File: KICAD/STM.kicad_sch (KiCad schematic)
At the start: 1 part, among them IC5 STM32F746BGT6

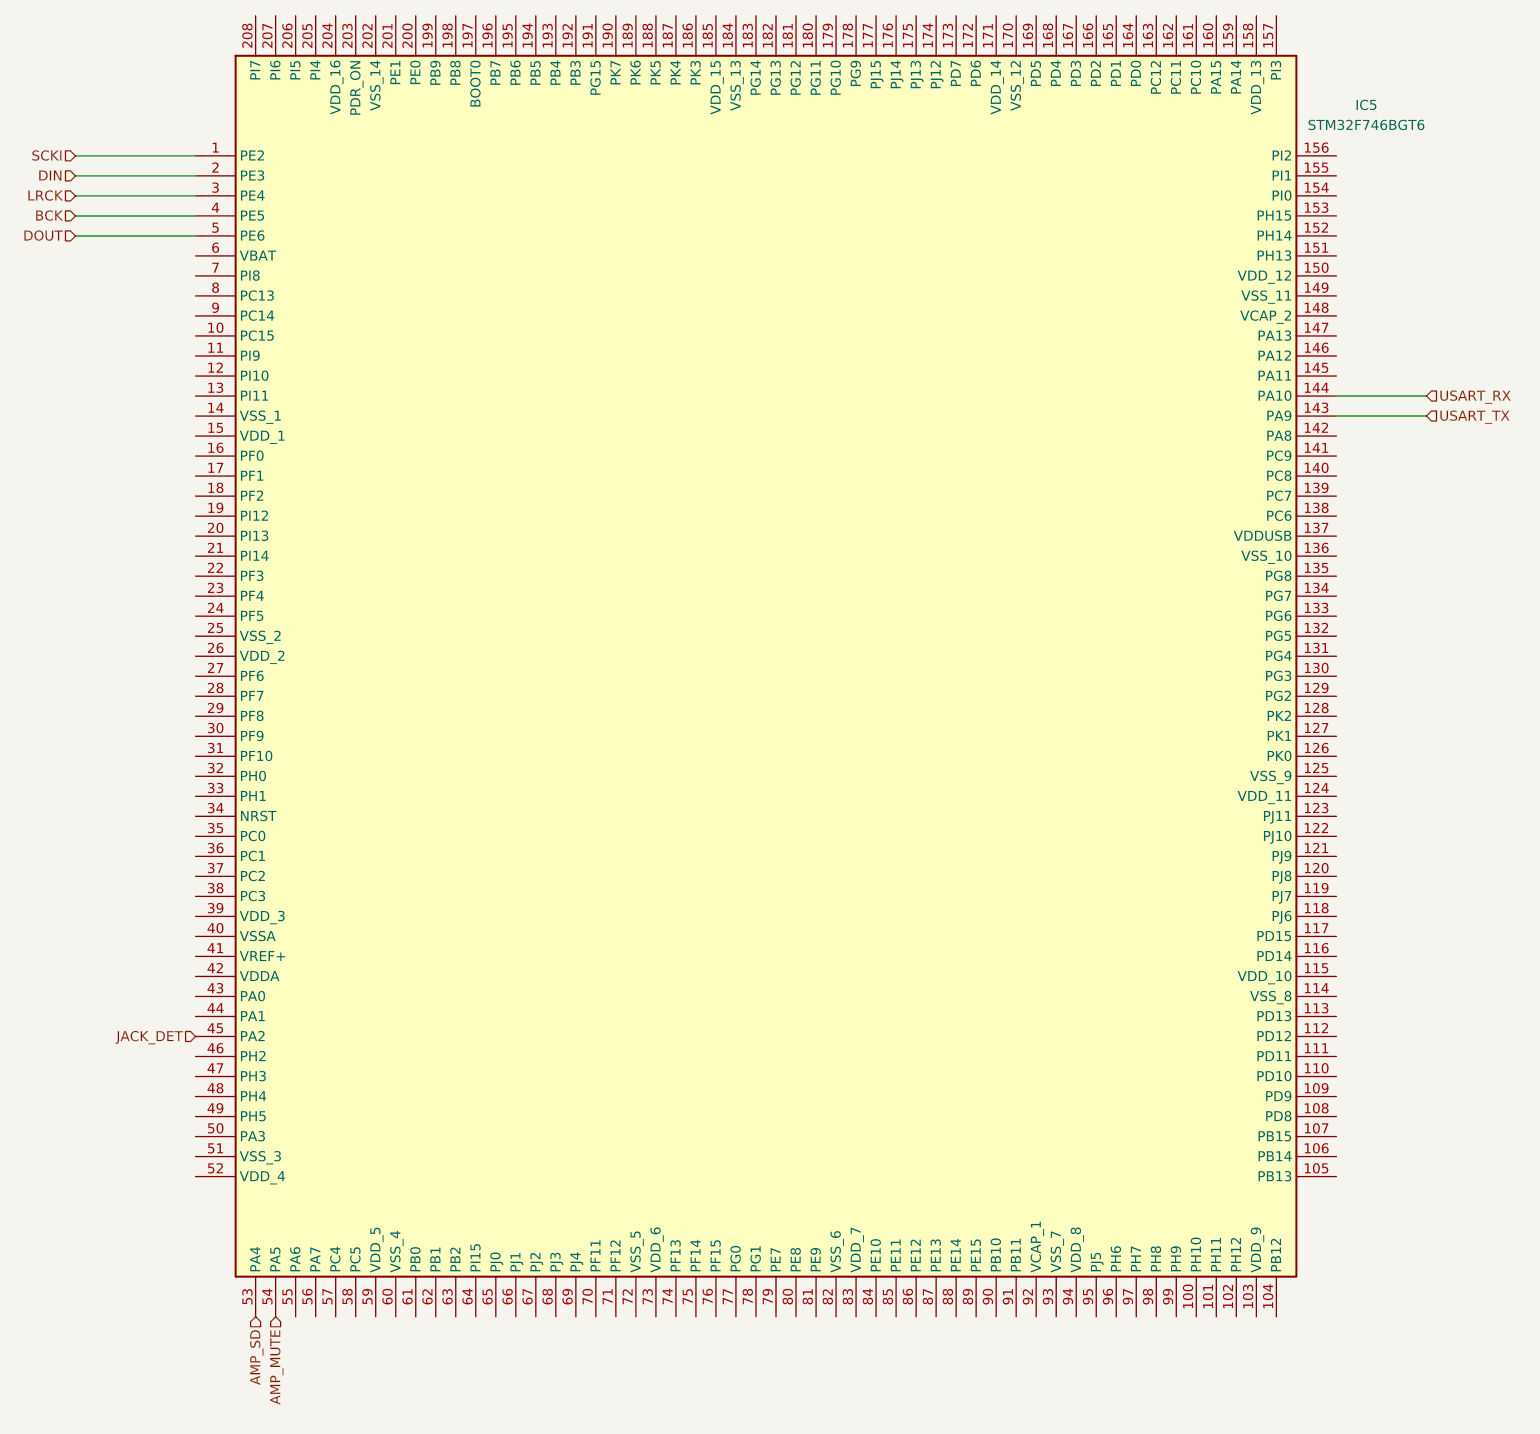
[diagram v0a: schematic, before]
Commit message: interface HM
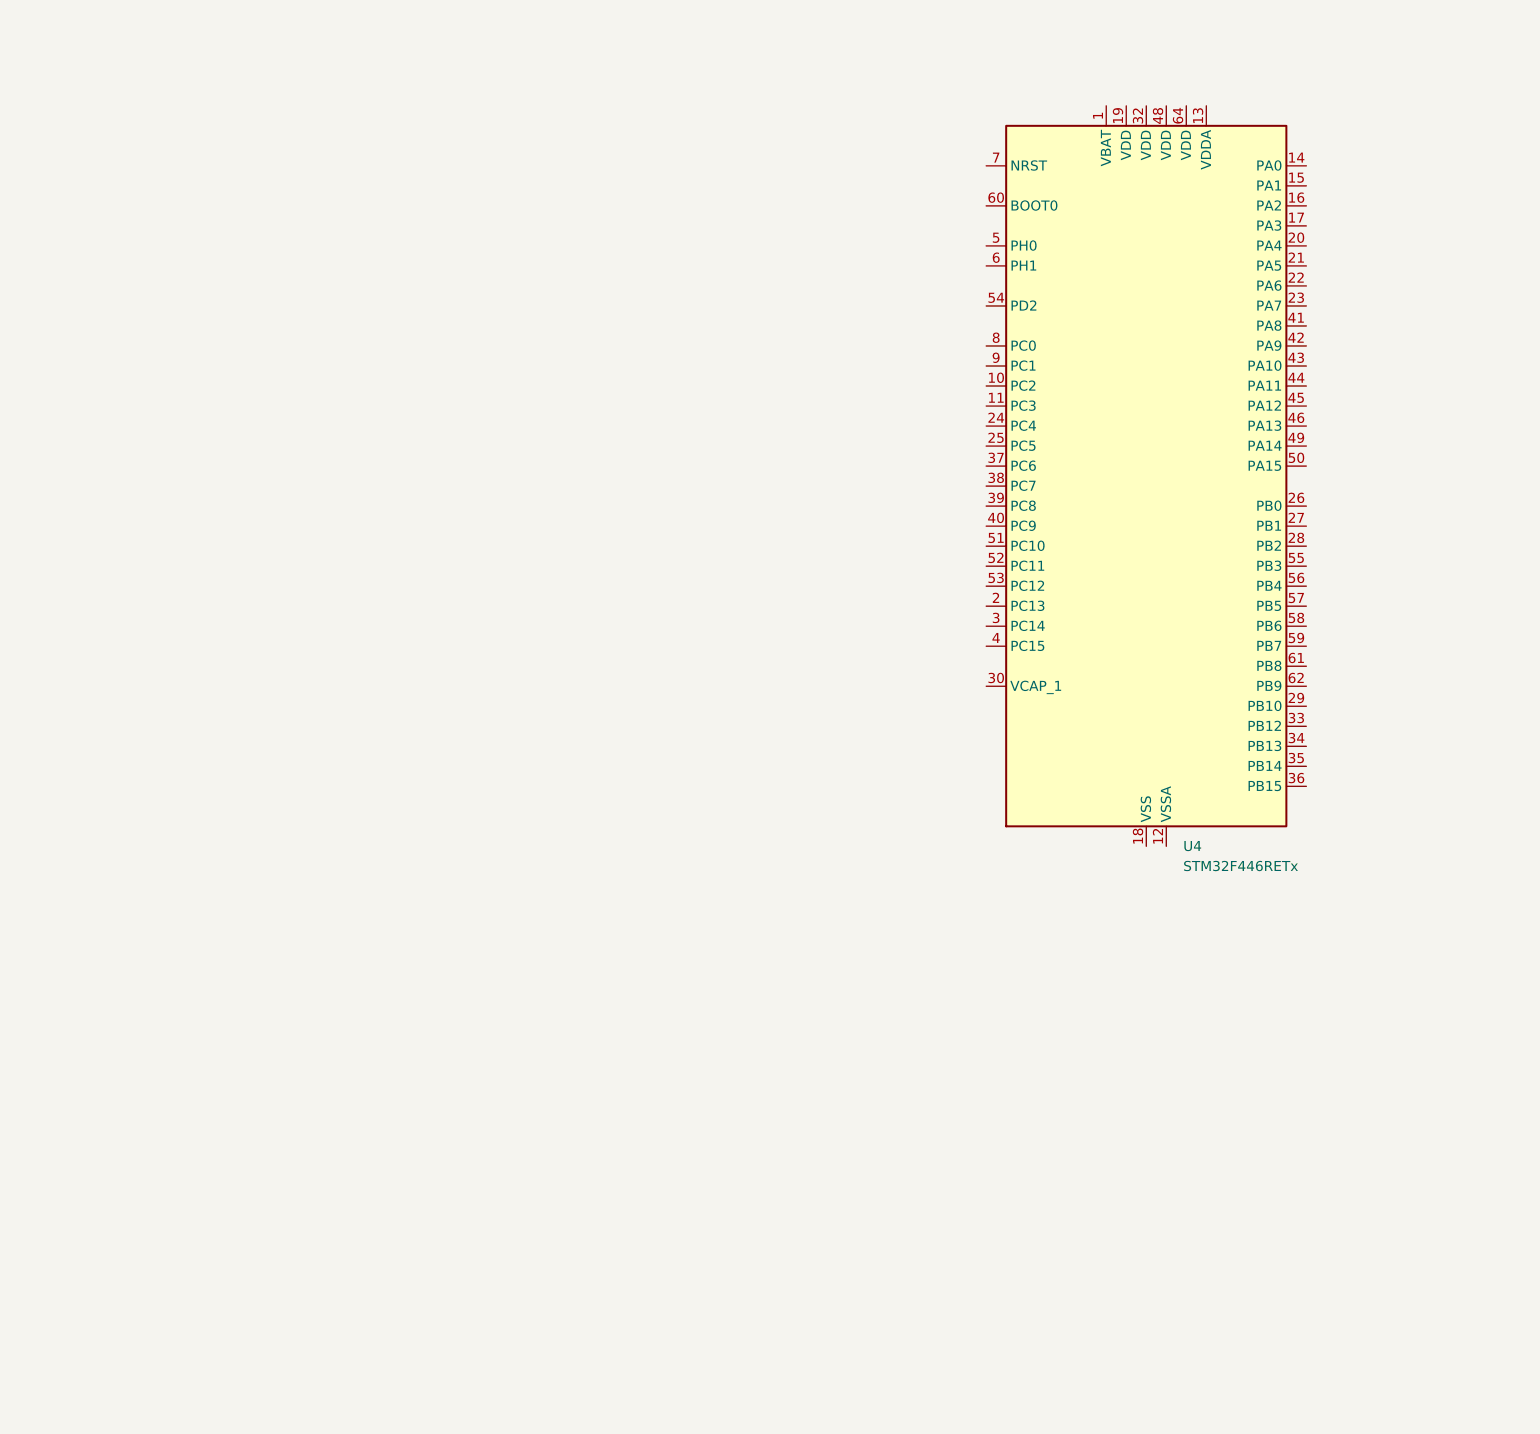
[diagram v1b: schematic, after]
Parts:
- removed IC5: STM32F746BGT6, footprints:STM32F746BGT6, symbol STM32F746BGT6:STM32F746BGT6
- added U4: STM32F446RETx, Package_QFP:LQFP-64_10x10mm_P0.5mm, symbol MCU_ST_STM32F4:STM32F446RETx
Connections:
- new net: U4.18 (VSS), U4.31 (VSS), U4.47 (VSS), U4.63 (VSS)
